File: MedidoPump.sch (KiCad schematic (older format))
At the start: 40 parts, among them J1 Flow_Fwd, J2 Flow_Rev, J3 Flow_Stop, J4 MultiplexConn, J5 OLED Disp, J6 Press_Sens, J7 MultiplexConn, J8 PwrButton, Q1 Q_NPN_EBC, SW1 SW_DPST, SW2 ~Boot, U1 BLE_FRIEND, U2 PowerButton, U3 LM7805_TO220, U4 HK3FF_RELAY, U5 ADS_1115, U6 Pololu18v17

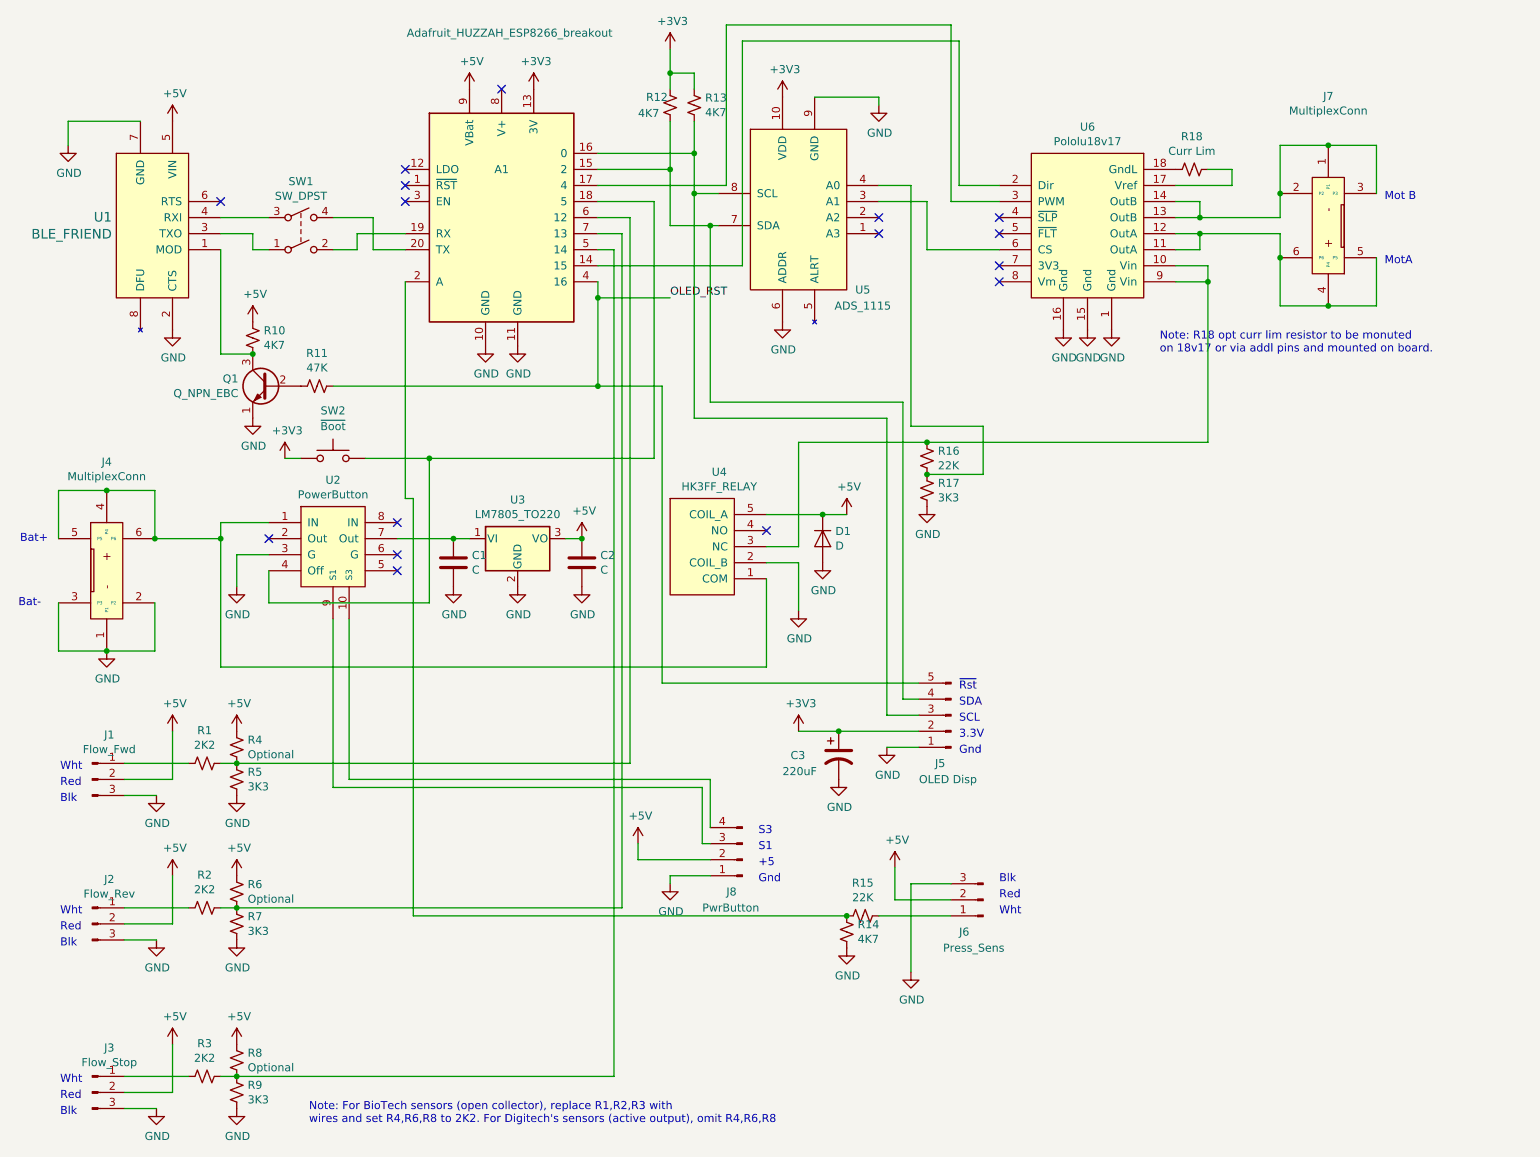
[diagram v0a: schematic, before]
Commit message: misc
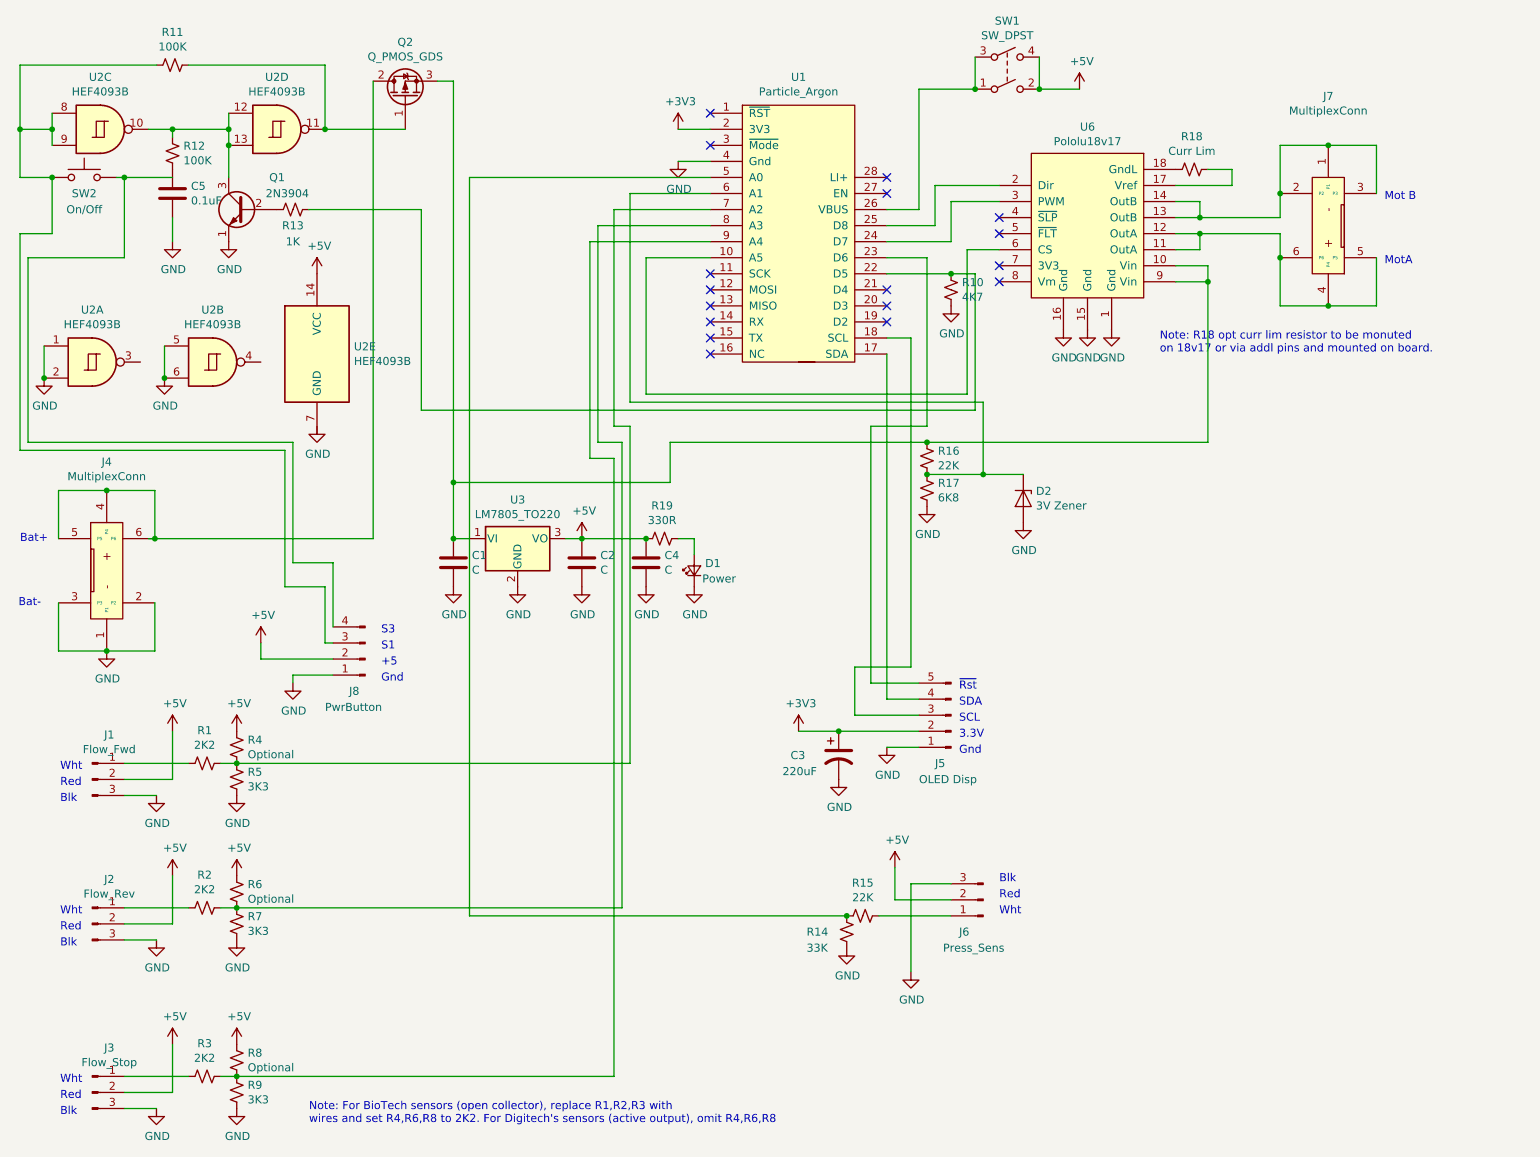
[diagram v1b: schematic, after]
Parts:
- removed A1: Adafruit_HUZZAH_ESP8266_breakout, Module:Adafruit_HUZZAH_ESP8266_breakout, symbol MCU_Module:Adafruit_HUZZAH_ESP8266_breakout
- removed D1: D, Diode_THT:D_5W_P10.16mm_Horizontal, symbol Device:D
- removed U1: BLE_FRIEND, MedidoFootprints:BLE_FRIEND, symbol medido:BLE_FRIEND
- removed U2: PowerButton, MedidoFootprints:PowerButton, symbol medido:PowerButton
- removed U4: HK3FF_RELAY, digikey-footprints:Relay_THT_G5LE-14, symbol MedidoPump-rescue:HK3FF_RELAY-medido
- removed U5: ADS_1115, MedidoFootprints:ADS_1115, symbol medido:ADS_1115
- added C4: C, Capacitor_THT:C_Disc_D12.0mm_W4.4mm_P7.75mm, symbol Device:C
- added C5: 0.1uF, Capacitor_THT:C_Disc_D12.0mm_W4.4mm_P7.75mm, symbol Device:C
- added D1: Power, LED_THT:LED_D3.0mm, symbol Device:LED_Small
- added D2: 3V Zener, Diode_THT:D_5W_P10.16mm_Horizontal, symbol Device:D_Zener
- added Q2: Q_PMOS_GDS, Package_TO_SOT_THT:TO-220-3_Vertical, symbol Device:Q_PMOS_GDS
- added R19: 330R, Resistor_THT:R_Axial_DIN0207_L6.3mm_D2.5mm_P10.16mm_Horizontal, symbol Device:R_Small_US
- added U1: Particle_Argon, MedidoFootprints:Particle_Argon, symbol medido:Particle_Argon
- added U2: HEF4093B, Package_DIP:DIP-14_W7.62mm, symbol 4xxx:HEF4093B
- Q1: value Q_NPN_EBC -> 2N3904; footprint digikey-footprints:SIP-3_P2.54mm -> Package_TO_SOT_THT:TO-126-3_Vertical
- R11: value 47K -> 100K
- R12: value 4K7 -> 100K
- R13: value 4K7 -> 1K
- R14: value 4K7 -> 33K
- R17: value 3K3 -> 6K8
- SW2: value ~Boot -> On/Off
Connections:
- net +3V3: now also U1.2 (3V3); no longer R12.1, R13.1, SW2.1
- net +5V: now also SW1.2, SW1.4, C4.1, R19.2, U2.14 (VCC); no longer R10.1
- net GND: now also R10.2, C4.2, C5.2, D1.1 (K), D2.2 (A), U1.4 (Gnd), U2.1, U2.2, U2.5, U2.6
- net at U6.2 (Dir): now also U1.25 (D8)
- net at J5.4 (Pin_4): now also U1.17 (SDA); no longer R12.2
- net at J5.3 (Pin_3): now also U1.18 (SCL); no longer R13.2
- net at U6.3 (PWM): now also U1.24 (D7)
- net at SW2.2: now also J8.4 (Pin_4)
- net at R14.1, R15.2: now also U1.5 (A0)
- net at R3.1, R8.2, R9.1: now also U1.9 (A4)
- net at R1.1, R4.2, R5.1: now also U1.7 (A2)
- net at R2.1, R6.2, R7.1: now also U1.8 (A3)
- net at Q1.3 (C): now also R12.1, U2.10, U2.12, U2.13; no longer R10.2
- net at SW1.1: now also SW1.3, U1.26 (VBUS)
- net at C1.1, U3.1 (VI): now also R16.1, U6.10 (Vin), U6.9 (Vin), Q2.3 (S)
- net at R11.2: now also J8.3 (Pin_3), SW2.1, U2.8, U2.9; no longer Q1.2 (B)
- net at R16.2, R17.1: now also D2.1 (K), U1.6 (A1)
- net at U6.6 (CS): now also U1.10 (A5)
- net at J4.4 (P4), J4.5 (P5), J4.6 (P6): now also Q2.2 (D)
- net OLED_RST: no longer names the net of J5.5 (Pin_5)
- net OLED_RST: now also U1.23 (D6); no longer R11.1
- new net: R10.1, R13.2, U1.22 (D5)
- new net: Q2.1 (G), R11.1, U2.11
- new net: C5.1, R12.2
- new net: Q1.2 (B), R13.1
- new net: D1.2 (A), R19.1
- no-connect marks 16 -> 17
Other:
- moved on the sheet: J8
